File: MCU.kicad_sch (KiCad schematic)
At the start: 21 parts, among them J1 USB_C_Receptacle_USB2.0, J5 Conn_01x05_Male, J5 Cortex_Debug, M4 Module-mega-mcu144-0.5, P10 Pad, P11 Pad, P12 Pad, P13 Pad, P14 Pad, P15 Pad, P3 Pad, P4 Pad, P5 Pad, P6 Pad, P7 Pad, P8 Pad, P9 Pad, U1 JDY-33

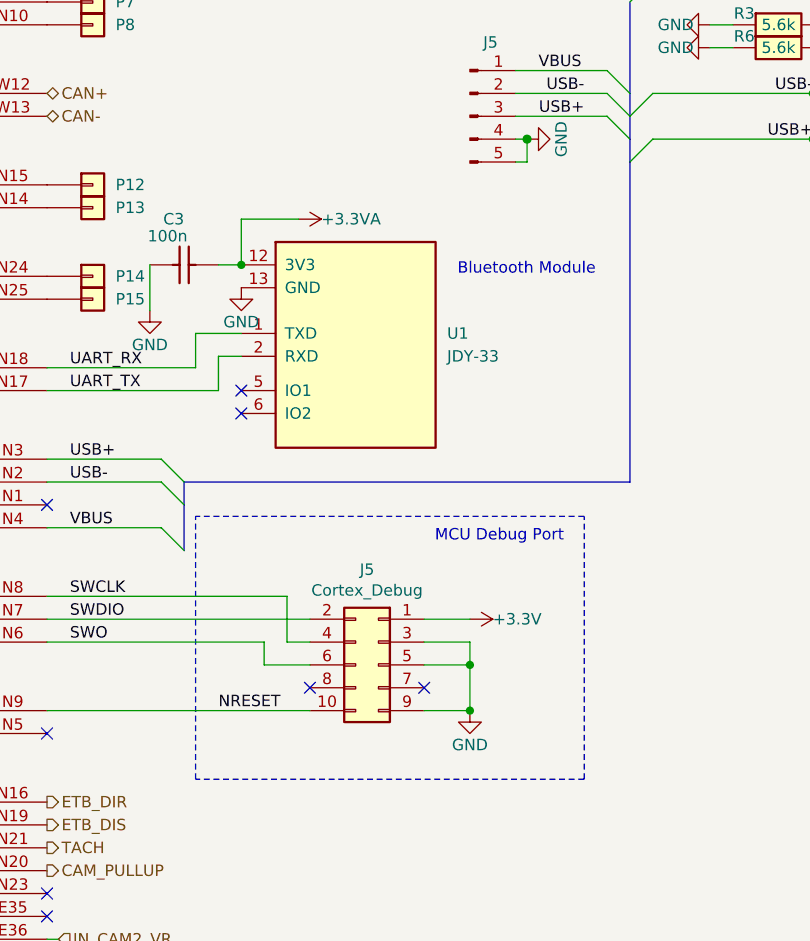
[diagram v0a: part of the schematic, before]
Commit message: Replace
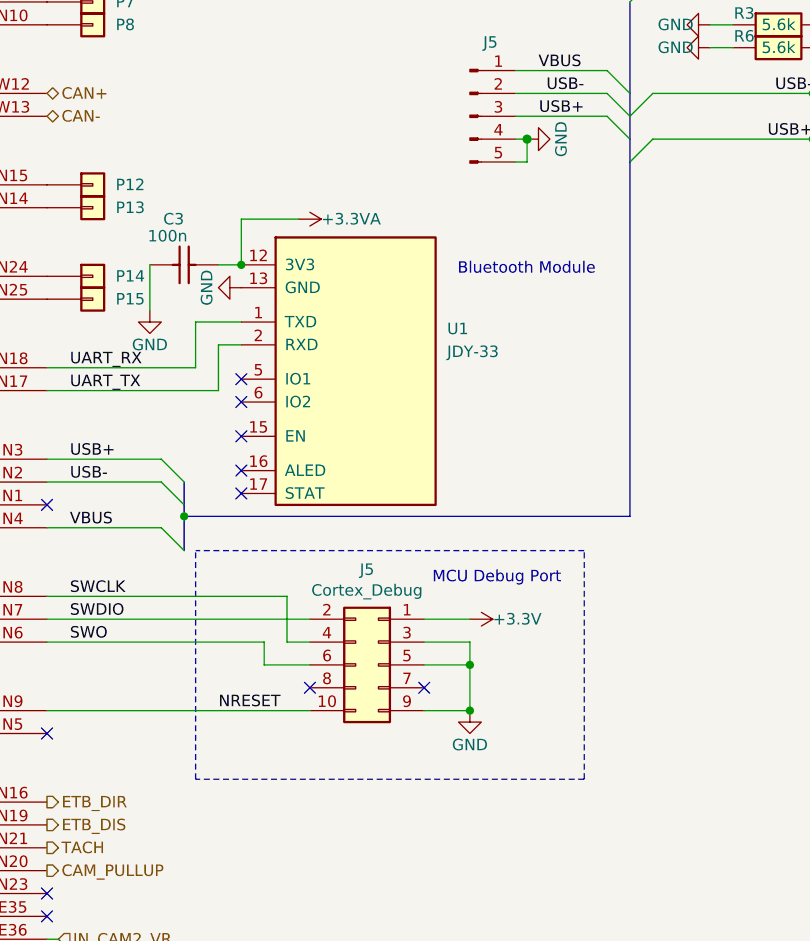
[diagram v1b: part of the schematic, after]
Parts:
- U1: footprint alphax-2ch:JDY-33 -> kicad6-libraries:JDY-33
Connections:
- no-connect marks 20 -> 23
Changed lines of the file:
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@@
   (junction (at 207.01 173.99) (diameter 0) (color 0 0 0 0)
+  )
+  (junction (at 175.26 152.4) (diameter 0) (color 0 0 0 0)
   )
   (junction (at 261.62 130.81) (diameter 1.016) (color 0 0 0 0)
@@
   (no_connect (at 160.02 214.63))
   (no_connect (at 160.02 77.47))
+  (no_connect (at 181.61 147.32))
+  (no_connect (at 181.61 149.86))
   (no_connect (at 189.23 171.45))
-  (no_connect (at 181.61 138.43))
+  (no_connect (at 181.61 137.16))
   (no_connect (at 201.93 171.45))
-  (no_connect (at 181.61 140.97))
+  (no_connect (at 181.61 139.7))
+  (no_connect (at 181.61 143.51))
   (no_connect (at 160.02 176.53))
   (no_connect (at 97.79 293.37))
@@
     (stroke (width 0) (type default))
   )
-  (bus (pts (xy 175.26 151.13) (xy 175.26 156.21))
-    (stroke (width 0) (type default))
-  )
-  (wire (pts (xy 176.53 135.89) (xy 176.53 132.08))
+  (bus (pts (xy 175.26 151.13) (xy 175.26 152.4))
+    (stroke (width 0) (type default))
+  )
+  (wire (pts (xy 176.53 135.89) (xy 176.53 130.81))
     (stroke (width 0) (type default))
   )
@@
     (stroke (width 0) (type default))
   )
+  (bus (pts (xy 175.26 152.4) (xy 175.26 156.21))
+    (stroke (width 0) (type default))
+  )
   (wire (pts (xy 245.11 107.95) (xy 245.11 105.41))
     (stroke (width 0) (type default))
@@
     (stroke (width 0) (type default))
   )
-  (polyline (pts (xy 176.53 181.61) (xy 176.53 152.4))
+  (polyline (pts (xy 176.53 181.61) (xy 176.53 156.21))
     (stroke (width 0) (type dash))
   )
@@
     (stroke (width 0) (type default))
   )
-  (wire (pts (xy 181.61 132.08) (xy 176.53 132.08))
-    (stroke (width 0) (type default))
-  )
-  (bus (pts (xy 224.79 113.03) (xy 224.79 148.59))
-    (stroke (width 0) (type default))
-  )
-  (polyline (pts (xy 219.71 152.4) (xy 176.53 152.4))
+  (wire (pts (xy 181.61 130.81) (xy 176.53 130.81))
+    (stroke (width 0) (type default))
+  )
+  (bus (pts (xy 224.79 113.03) (xy 224.79 152.4))
+    (stroke (width 0) (type default))
+  )
+  (polyline (pts (xy 219.71 156.21) (xy 176.53 156.21))
     (stroke (width 0) (type dash))
   )
@@
     (stroke (width 0) (type solid))
   )
-  (wire (pts (xy 179.07 138.43) (xy 179.07 134.62))
+  (wire (pts (xy 179.07 138.43) (xy 179.07 133.35))
     (stroke (width 0) (type default))
   )
@@
     (stroke (width 0) (type default))
   )
+  (bus (pts (xy 175.26 152.4) (xy 224.79 152.4))
+    (stroke (width 0) (type default))
+  )
   (wire (pts (xy 207.01 166.37) (xy 207.01 168.91))
     (stroke (width 0) (type default))
   )
-  (polyline (pts (xy 219.71 181.61) (xy 219.71 152.4))
+  (polyline (pts (xy 219.71 181.61) (xy 219.71 156.21))
     (stroke (width 0) (type dash))
   )
@@
   )
   (wire (pts (xy 85.09 81.28) (xy 97.79 81.28))
-    (stroke (width 0) (type default))
-  )
-  (bus (pts (xy 224.79 148.59) (xy 175.26 148.59))
     (stroke (width 0) (type default))
   )
@@
     (stroke (width 0) (type default))
   )
-  (wire (pts (xy 179.07 134.62) (xy 181.61 134.62))
+  (wire (pts (xy 179.07 133.35) (xy 181.61 133.35))
     (stroke (width 0) (type default))
   )
@@
     (effects (font (size 1.27 1.27)) (justify right bottom))
   )
-  (text "MCU Debug Port" (at 217.4546 155.3723 0)
+  (text "MCU Debug Port" (at 217.17 160.02 0)
     (effects (font (size 1.27 1.27)) (justify right bottom))
   )
@@
     )
   )
-  (symbol (lib_id "JDY-33:JDY-33") (at 185.42 133.858 0) (unit 1)
-    (in_bom yes) (on_board yes) (dnp no)
-    (property "Reference" "U1" (at 204.47 132.08 0)
+  (symbol (lib_id "JDY-33:JDY-33") (at 185.42 133.35 0) (unit 1)
+    (in_bom yes) (on_board yes) (dnp no)
+    (property "Reference" "U1" (at 204.47 131.572 0)
       (effects (font (size 1.27 1.27)) (justify left))
     )
-    (property "Value" "JDY-33" (at 204.47 134.62 0)
+    (property "Value" "JDY-33" (at 204.47 134.112 0)
       (effects (font (size 1.27 1.27)) (justify left))
     )
-    (property "Footprint" "alphax-2ch:JDY-33" (at 185.42 133.858 0)
+    (property "Footprint" "kicad6-libraries:JDY-33" (at 185.42 133.35 0)
       (effects (font (size 1.27 1.27)) (justify left bottom) hide)
     )
-    (property "Datasheet" "https://datasheet.lcsc.com/lcsc/2106070033_QIACHIP-WL9981TC_C2689544.pdf" (at 185.42 133.858 0)
+    (property "Datasheet" "https://datasheet.lcsc.com/lcsc/2106070033_QIACHIP-WL9981TC_C2689544.pdf" (at 185.42 133.35 0)
       (effects (font (size 1.27 1.27)) (justify left bottom) hide)
     )
-    (property "LCSC" "" (at 185.42 133.858 0)
-      (effects (font (size 1.27 1.27)) hide)
-    )
-    (property "PARTREV" "v1.0" (at 185.42 133.858 0)
+    (property "LCSC" "" (at 185.42 133.35 0)
+      (effects (font (size 1.27 1.27)) hide)
+    )
+    (property "PARTREV" "v1.0" (at 185.42 133.35 0)
       (effects (font (size 1.27 1.27)) (justify left bottom) hide)
     )
-    (property "MF" "HuiCheng" (at 185.42 133.858 0)
+    (property "MF" "HuiCheng" (at 185.42 133.35 0)
       (effects (font (size 1.27 1.27)) (justify left bottom) hide)
     )
-    (property "STANDARD" "Manufacturer Recommendations" (at 185.42 133.858 0)
+    (property "STANDARD" "Manufacturer Recommendations" (at 185.42 133.35 0)
       (effects (font (size 1.27 1.27)) (justify left bottom) hide)
     )
@@
     (pin "5")
     (pin "6")
+    (pin "16")
+    (pin "17")
+    (pin "15")
     (instances
       (project "alphax_4ch"
@@
     )
   )
-  (symbol (lib_id "power:GND") (at 181.61 127 0) (unit 1)
-    (in_bom yes) (on_board yes) (dnp no)
-    (property "Reference" "#PWR079" (at 181.61 133.35 0)
-      (effects (font (size 1.27 1.27)) hide)
-    )
-    (property "Value" "GND" (at 181.61 130.81 0)
-      (effects (font (size 1.27 1.27)))
-    )
+  (symbol (lib_id "power:GND") (at 181.61 127 270) (unit 1)
+    (in_bom yes) (on_board yes) (dnp no)
+    (property "Reference" "#PWR079" (at 175.26 127 0)
+      (effects (font (size 1.27 1.27)) hide)
+    )
+    (property "Value" "GND" (at 177.8 127 0)
+      (effects (font (size 1.27 1.27)))
+    )
